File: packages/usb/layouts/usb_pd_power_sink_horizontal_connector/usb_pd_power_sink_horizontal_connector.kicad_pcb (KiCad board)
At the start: 2 copper layers, 8 parts, among them U2 2.9V

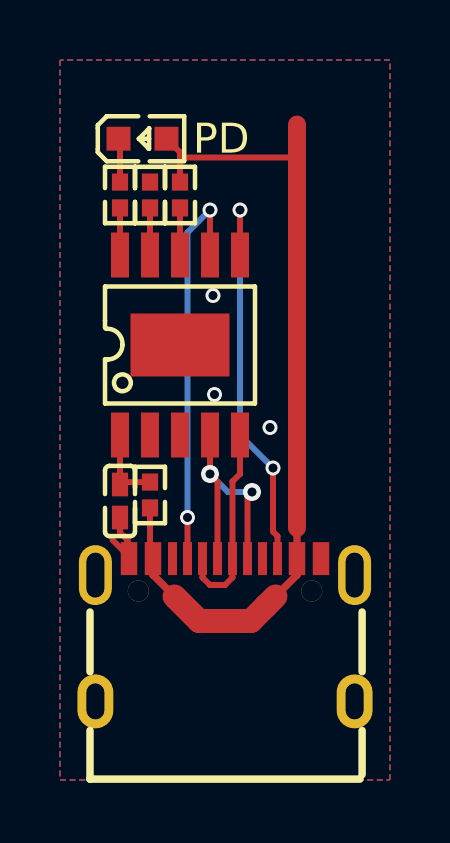
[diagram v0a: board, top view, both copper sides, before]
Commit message: WIP update usb
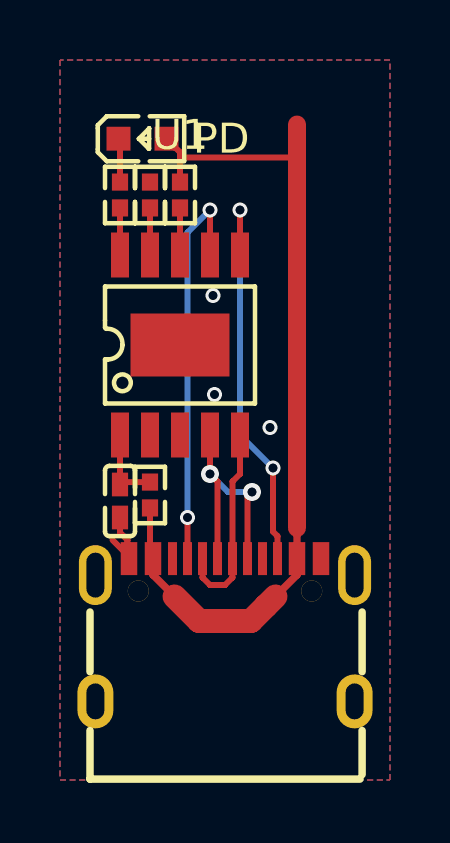
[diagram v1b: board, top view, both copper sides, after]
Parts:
- C1: value 1µF ±10% 16V X5R -> 1µF ±10% 25V X5R; footprint atopile:C0402-b3ef17 -> Samsung_Electro_Mechanics_CL05A105KA5NQNC:C0402
- R1, R2, R4: footprint atopile:R0402-56259e -> UNI_ROYAL_0402WGF1002TCE:R0402
- R3: footprint atopile:R0402-56259e -> UNI_ROYAL_0402WGF1001TCE:R0402
- U1: footprint atopile:ESSOP-10_L4.9-W3.9-P1.0-LS6.0-TL-EP-20a8ca -> WCH_CH224K:ESSOP-10_L4.9-W3.9-P1.0-LS6.0-TL-EP
- U2: footprint lib:LED0603-RD -> Hubei_KENTO_Elec_Blue_light_0603:LED0603-RD
- X1: footprint atopile:USB-C-SMD_TYPE-C-6PIN-2MD-073-1d78f0 -> SHOU_HAN_TYPE_C_16PIN_2MD_073:USB-C-SMD_TYPE-C-6PIN-2MD-073
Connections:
- U1 pad 2: pd_trigger.controller-line -> pd_trigger.controller-line-1
- U1 pad 3: pd_trigger.controller-line-1 -> pd_trigger.controller-line
- U1 pad 4: line-1 -> line-4
- U1 pad 6: line -> line-5
- X1 pad : (no net) -> net
- X1 pad 10: line -> line-5
- X1 pad 3: line-4 -> line
- X1 pad 6: line-1 -> line-4
- X1 pad 8: line-1 -> line-4
- X1 pad 9: line-5 -> line-1
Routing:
- net line-5: track 0.00 -> 13.6 mm, vias 0 -> 2
- net line: track 13.6 -> 0.00 mm, vias 2 -> 0
- net line-4: track 0.00 -> 8.15 mm, vias 0 -> 2
- net line-1: track 8.15 -> 0.00 mm, vias 2 -> 0
